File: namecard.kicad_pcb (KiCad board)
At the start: 2 copper layers, 85.6 x 54 mm, 41 parts, among them J1 Conn_01x24, J2 Conn_01x05, Q1 AO3400A, U1 STM32G030K6Tx, U2 ST25DV04K-IER8C3

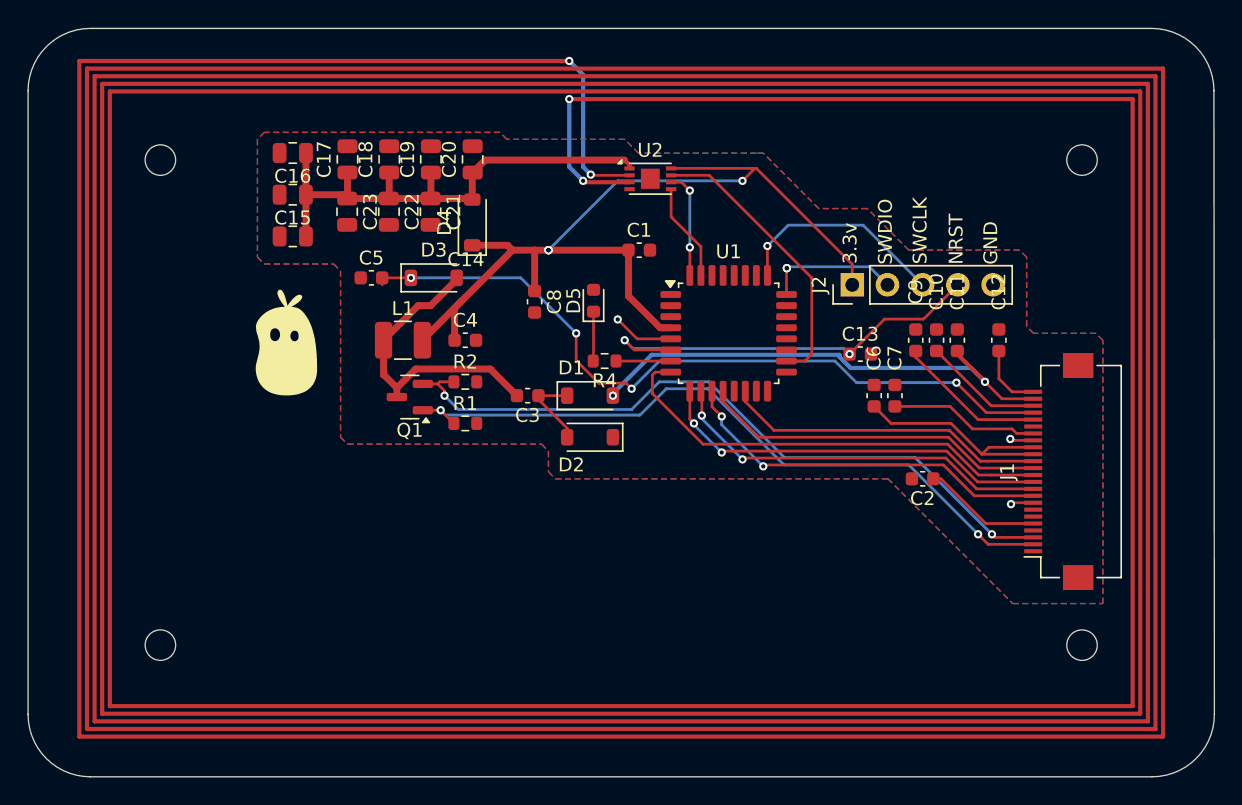
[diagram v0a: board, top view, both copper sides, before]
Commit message: v2 production
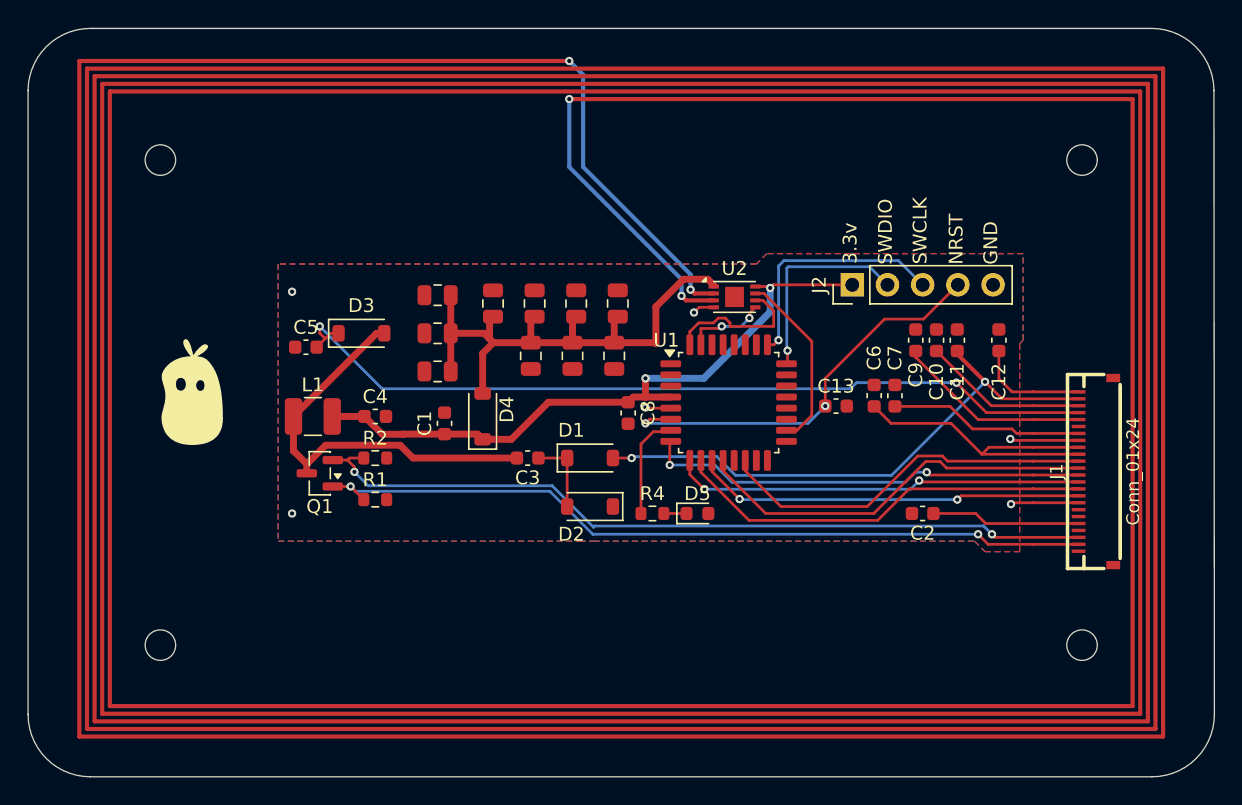
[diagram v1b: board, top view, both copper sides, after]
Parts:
- J1: footprint Connector_FFC-FPC:Hirose_FH12-24S-0.5SH_1x24-1MP_P0.50mm_Horizontal -> Connector:FFC-SMD_24P-P0.50_FH34SRJ-24S-0.5SH
- moved C1 18.8 mm to (122.5, 94.5), turned to 90 degrees
- moved D5 17.1 mm to (140.8, 101.0), turned to 0 degrees
- moved C22 16.8 mm to (131.7, 89.6)
- moved C21 16.8 mm to (134.7, 89.6)
- moved C23 16.8 mm to (128.7, 89.6)
- moved C17 14.8 mm to (126.0, 85.8)
- moved C18 14.8 mm to (129.0, 85.8)
- moved C19 14.8 mm to (132.0, 85.8)
- moved C20 14.8 mm to (135.0, 85.8)
- moved C16 14.6 mm to (122.0, 85.2)
- moved C15 14.5 mm to (122.0, 88.0)
- moved C14 14.3 mm to (122.0, 90.8)
- moved D4 14.0 mm to (125.2, 94.0)
- moved R4 11.5 mm to (137.5, 101.0), turned to 0 degrees
- moved C8 10.5 mm to (135.8, 93.8)
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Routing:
- net /EXT_3V3: track 68.7 -> 47.6 mm, vias 4 -> 2
- net Net-(U2-AC0): track 1244.1 -> 1264.7 mm
- net Net-(D3-A): track 21.8 -> 29.7 mm
- net /NFC_INT: track 20.7 -> 13.1 mm
- net Net-(J1-Pin_15): track 16.8 -> 23.4 mm
- net /PREVGH: track 54.7 -> 60.7 mm, vias 4 -> 2
- net /GDR: track 51.1 -> 57.0 mm
- net /RESE: track 51.7 -> 57.6 mm
- net GND: track 7.74 -> 13.3 mm, vias 3 -> 6
- net /SWDIO: track 9.75 -> 14.8 mm, vias 2 -> 1
- net /PREVGL: track 36.1 -> 40.6 mm
- net /SPI_SCK: track 25.1 -> 29.4 mm
- net /SPI_MOSI: track 23.3 -> 27.5 mm
- net Net-(U1-PA0): track 3.95 -> 7.57 mm
- net Net-(J1-Pin_22): track 8.61 -> 11.9 mm
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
